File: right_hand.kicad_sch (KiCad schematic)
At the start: 54 parts, among them J1 AudioJack4, J2 SWD, J3 USB_C_Receptacle_USB2.0, SW1 Boot, U1 W25Q128JVS, U2 RP2040, U3 PRTR5V0U2X, U4 XC6206PxxxMR, Y1 12MHz

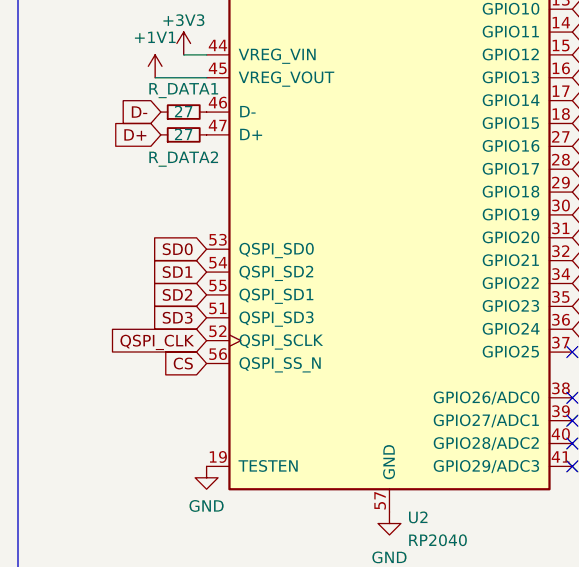
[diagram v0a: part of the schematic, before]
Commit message: final, working
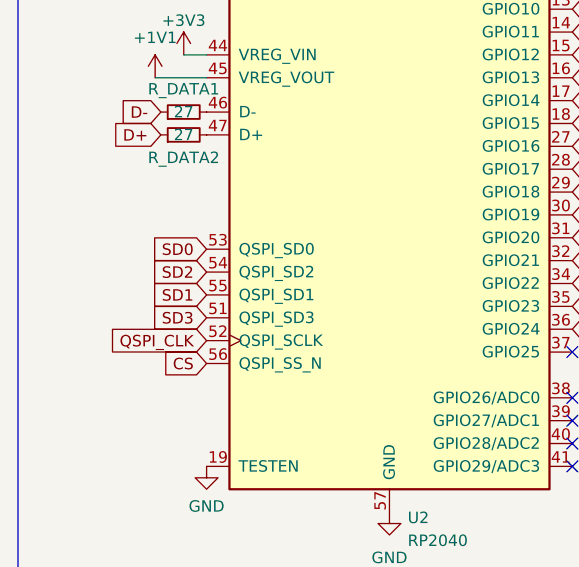
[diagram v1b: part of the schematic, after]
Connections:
- net SD1: now also U2.55 (QSPI_SD1); no longer U2.54 (QSPI_SD2)
- net SD2: now also U2.54 (QSPI_SD2); no longer U2.55 (QSPI_SD1)
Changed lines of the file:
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@@
     )
   )
-  (global_label "SD1" (shape input) (at 33.655 90.805 180) (fields_autoplaced)
+  (global_label "SD1" (shape input) (at 33.655 93.345 180) (fields_autoplaced)
+    (effects (font (size 1.27 1.27)) (justify right))
+    (property "Intersheetrefs" "${INTERSHEET_REFS}" (at 27.5529 93.2656 0)
+      (effects (font (size 1.27 1.27)) (justify right) hide)
+    )
+  )
+  (global_label "SD2" (shape input) (at 33.655 90.805 180) (fields_autoplaced)
     (effects (font (size 1.27 1.27)) (justify right))
     (property "Intersheetrefs" "${INTERSHEET_REFS}" (at 27.5529 90.7256 0)
       (effects (font (size 1.27 1.27)) (justify right) hide)
     )
-  )
-  (global_label "SD2" (shape input) (at 33.655 93.345 180) (fields_autoplaced)
-    (effects (font (size 1.27 1.27)) (justify right))
-    (property "Intersheetrefs" "${INTERSHEET_REFS}" (at 27.5529 93.2656 0)
-      (effects (font (size 1.27 1.27)) (justify right) hide)
-    )

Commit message: replace trrs
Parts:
- MX1, MX10, MX11, MX12, MX13, MX14, MX15, MX16, MX17, MX18, MX2, MX3, MX4, MX5, MX6, MX7, MX8, MX9: footprint parts:mx_1u -> parts:Kailh_socket_MX
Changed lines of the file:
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@@
       (effects (font (size 1.27 1.27)))
     )
-    (property "Footprint" "parts:mx_1u" (at 212.725 45.085 0)
+    (property "Footprint" "parts:Kailh_socket_MX" (at 212.725 45.085 0)
       (effects (font (size 1.27 1.27)) hide)
     )
@@
       (effects (font (size 1.27 1.27)))
     )
-    (property "Footprint" "parts:mx_1u" (at 250.825 26.035 0)
+    (property "Footprint" "parts:Kailh_socket_MX" (at 250.825 26.035 0)
       (effects (font (size 1.27 1.27)) hide)
     )
@@
       (effects (font (size 1.27 1.27)))
     )
-    (property "Footprint" "parts:mx_1u" (at 225.425 83.185 0)
+    (property "Footprint" "parts:Kailh_socket_MX" (at 225.425 83.185 0)
       (effects (font (size 1.27 1.27)) hide)
     )
@@
       (effects (font (size 1.27 1.27)))
     )
-    (property "Footprint" "parts:mx_1u" (at 263.525 64.135 0)
+    (property "Footprint" "parts:Kailh_socket_MX" (at 263.525 64.135 0)
       (effects (font (size 1.27 1.27)) hide)
     )
@@
       (effects (font (size 1.27 1.27)))
     )
-    (property "Footprint" "parts:mx_1u" (at 225.425 45.085 0)
+    (property "Footprint" "parts:Kailh_socket_MX" (at 225.425 45.085 0)
       (effects (font (size 1.27 1.27)) hide)
     )
@@
       (effects (font (size 1.27 1.27)))
     )
-    (property "Footprint" "parts:mx_1u" (at 263.525 45.085 0)
+    (property "Footprint" "parts:Kailh_socket_MX" (at 263.525 45.085 0)
       (effects (font (size 1.27 1.27)) hide)
     )
@@
       (effects (font (size 1.27 1.27)))
     )
-    (property "Footprint" "parts:mx_1u" (at 263.525 26.035 0)
+    (property "Footprint" "parts:Kailh_socket_MX" (at 263.525 26.035 0)
       (effects (font (size 1.27 1.27)) hide)
     )
@@
       (effects (font (size 1.27 1.27)))
     )
-    (property "Footprint" "parts:mx_1u" (at 212.725 26.035 0)
+    (property "Footprint" "parts:Kailh_socket_MX" (at 212.725 26.035 0)
       (effects (font (size 1.27 1.27)) hide)
     )
@@
       (effects (font (size 1.27 1.27)))
     )
-    (property "Footprint" "parts:mx_1u" (at 238.125 83.185 0)
+    (property "Footprint" "parts:Kailh_socket_MX" (at 238.125 83.185 0)
       (effects (font (size 1.27 1.27)) hide)
     )
@@
       (effects (font (size 1.27 1.27)))
     )
-    (property "Footprint" "parts:mx_1u" (at 238.125 45.085 0)
+    (property "Footprint" "parts:Kailh_socket_MX" (at 238.125 45.085 0)
       (effects (font (size 1.27 1.27)) hide)
     )
@@
       (effects (font (size 1.27 1.27)))
     )
-    (property "Footprint" "parts:mx_1u" (at 225.425 64.135 0)
+    (property "Footprint" "parts:Kailh_socket_MX" (at 225.425 64.135 0)
       (effects (font (size 1.27 1.27)) hide)
     )
@@
       (effects (font (size 1.27 1.27)))
     )
-    (property "Footprint" "parts:mx_1u" (at 212.725 83.185 0)
+    (property "Footprint" "parts:Kailh_socket_MX" (at 212.725 83.185 0)
       (effects (font (size 1.27 1.27)) hide)
     )
@@
       (effects (font (size 1.27 1.27)))
     )
-    (property "Footprint" "parts:mx_1u" (at 250.825 64.135 0)
+    (property "Footprint" "parts:Kailh_socket_MX" (at 250.825 64.135 0)
       (effects (font (size 1.27 1.27)) hide)
     )
@@
       (effects (font (size 1.27 1.27)))
     )
-    (property "Footprint" "parts:mx_1u" (at 238.125 26.035 0)
+    (property "Footprint" "parts:Kailh_socket_MX" (at 238.125 26.035 0)
       (effects (font (size 1.27 1.27)) hide)
     )
@@
       (effects (font (size 1.27 1.27)))
     )
-    (property "Footprint" "parts:mx_1u" (at 225.425 26.035 0)
+    (property "Footprint" "parts:Kailh_socket_MX" (at 225.425 26.035 0)
       (effects (font (size 1.27 1.27)) hide)
     )
@@
       (effects (font (size 1.27 1.27)))
     )
-    (property "Footprint" "parts:mx_1u" (at 250.825 45.085 0)
+    (property "Footprint" "parts:Kailh_socket_MX" (at 250.825 45.085 0)
       (effects (font (size 1.27 1.27)) hide)
     )
@@
       (effects (font (size 1.27 1.27)))
     )
-    (property "Footprint" "parts:mx_1u" (at 212.725 64.135 0)
+    (property "Footprint" "parts:Kailh_socket_MX" (at 212.725 64.135 0)
       (effects (font (size 1.27 1.27)) hide)
     )
@@
       (effects (font (size 1.27 1.27)))
     )
-    (property "Footprint" "parts:mx_1u" (at 238.125 64.135 0)
-      (effects (font (size 1.27 1.27)) hide)
-    )
+    (property "Footprint" "parts:Kailh_socket_MX" (at 238.125 64.135 0)
+      (effects (font (size 1.27 1.27)) hide)
+    )
